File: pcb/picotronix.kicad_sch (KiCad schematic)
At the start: 27 parts, among them J1 Conn_02x04_Odd_Even, J2 Conn_02x04_Odd_Even, J3 DEBUG, J4 DB25_Male, U1 Pico, U2 LSF0204DPWR, U3 DAC7562SDGST, U4 ADA4891-3

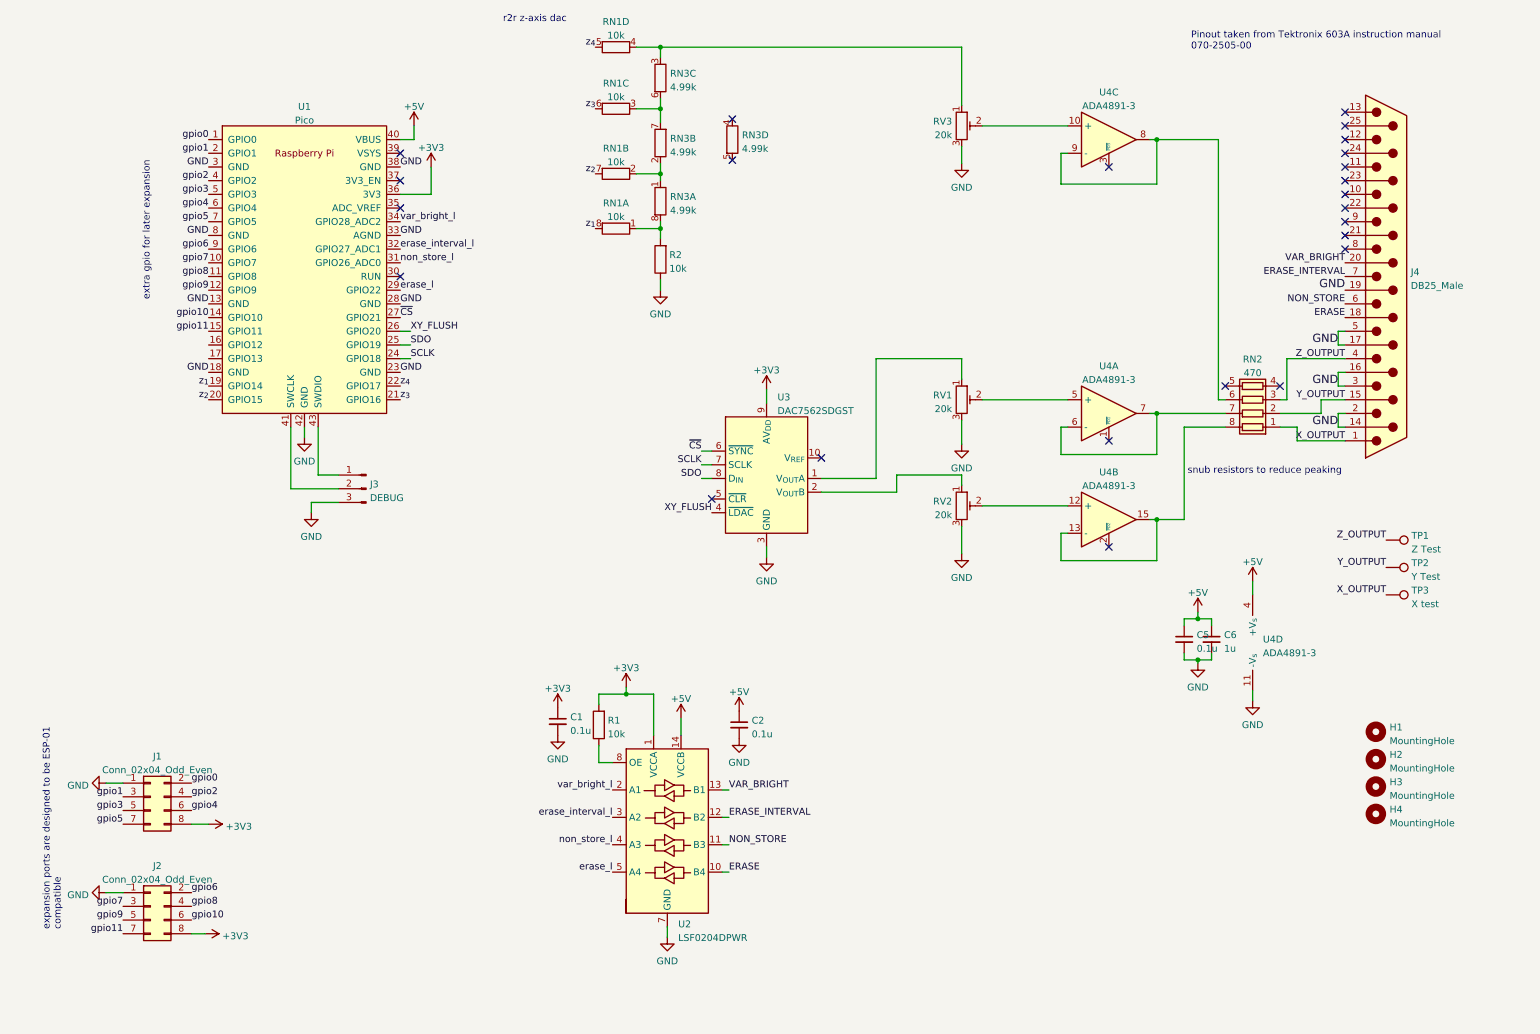
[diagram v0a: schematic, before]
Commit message: pcb rev2 routed
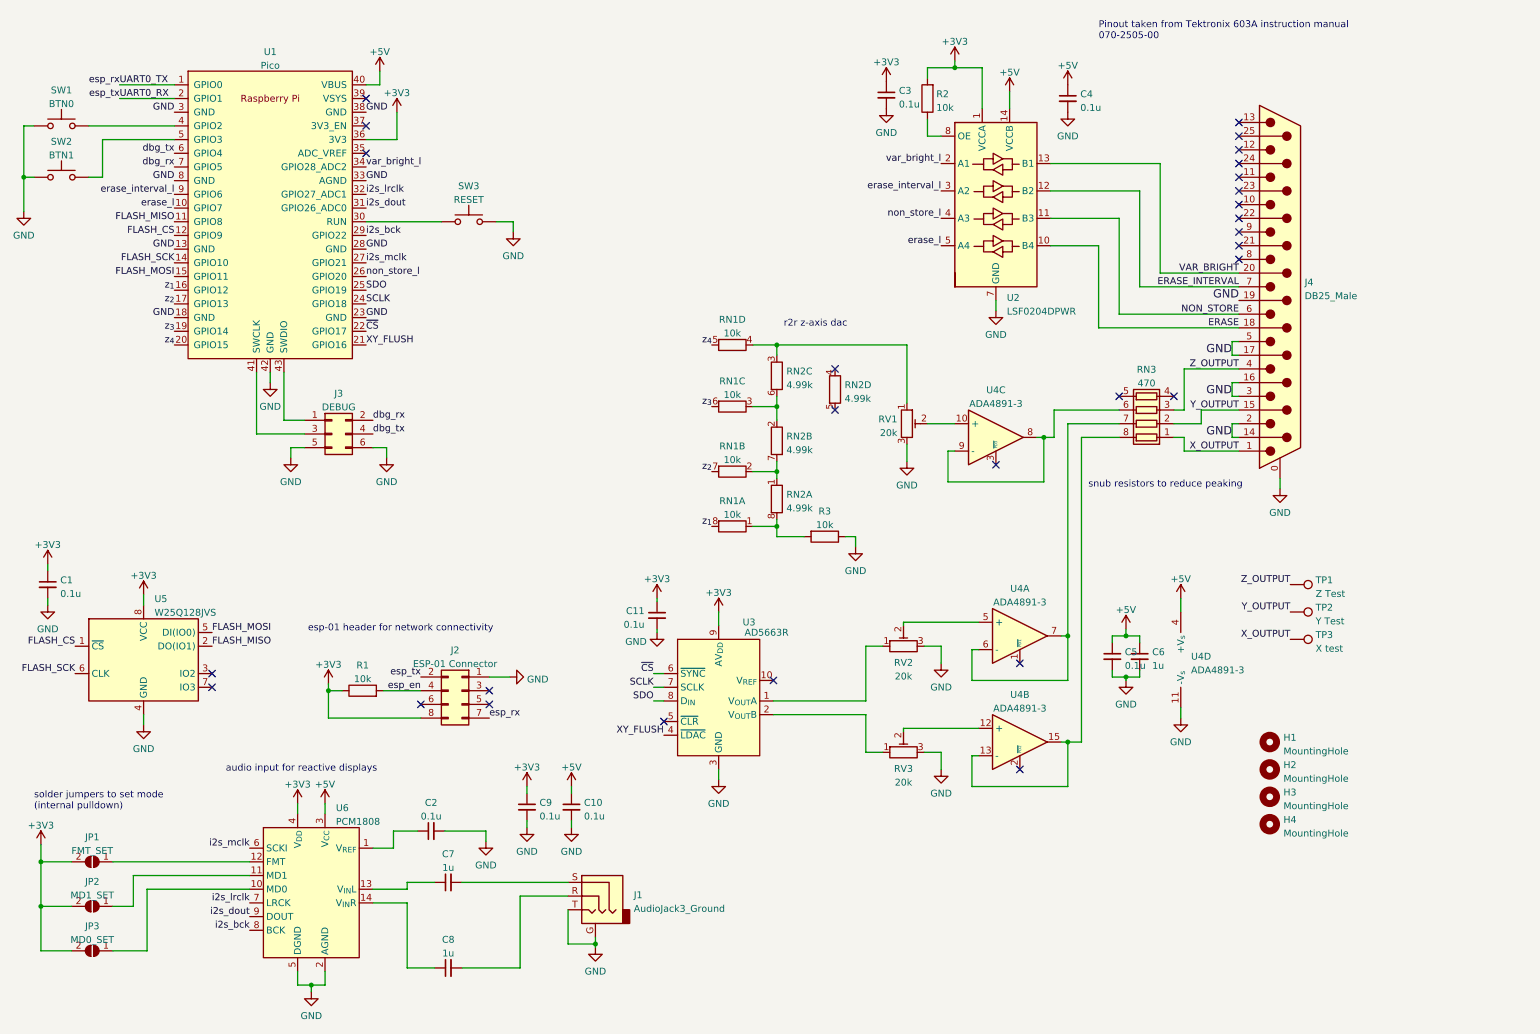
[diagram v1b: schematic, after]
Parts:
- removed J2: Conn_02x04_Odd_Even, Connector_PinSocket_2.54mm:PinSocket_2x04_P2.54mm_Vertical, symbol Connector_Generic:Conn_02x04_Odd_Even
- removed J3: DEBUG, Connector_PinHeader_2.54mm:PinHeader_1x03_P2.54mm_Vertical, symbol Connector:Conn_01x03_Male
- added C1, C10, C11, C2, C9: 0.1u, Capacitor_SMD:C_0603_1608Metric_Pad1.08x0.95mm_HandSolder, symbol Device:C_Small
- added C7, C8: 1u, Capacitor_SMD:C_0603_1608Metric_Pad1.08x0.95mm_HandSolder, symbol Device:C_Small
- added J1: AudioJack3_Ground, Connector_Audio:Jack_3.5mm_CUI_SJ-3524-SMT_Horizontal, symbol Connector:AudioJack3_Ground
- added J3: DEBUG, Connector_PinHeader_2.54mm:PinHeader_2x03_P2.54mm_Vertical, symbol Connector_Generic:Conn_02x03_Odd_Even
- added JP1: FMT_SET, Jumper:SolderJumper-2_P1.3mm_Open_TrianglePad1.0x1.5mm, symbol Jumper:SolderJumper_2_Open
- added JP2: MD1_SET, Jumper:SolderJumper-2_P1.3mm_Open_TrianglePad1.0x1.5mm, symbol Jumper:SolderJumper_2_Open
- added JP3: MD0_SET, Jumper:SolderJumper-2_P1.3mm_Open_TrianglePad1.0x1.5mm, symbol Jumper:SolderJumper_2_Open
- added R1: 10k, Resistor_SMD:R_0603_1608Metric_Pad0.98x0.95mm_HandSolder, symbol Device:R
- added SW1: BTN0, Button_Switch_SMD:SW_SPST_TL3305A, symbol Switch:SW_Push
- added SW2: BTN1, Button_Switch_SMD:SW_SPST_TL3305A, symbol Switch:SW_Push
- added SW3: RESET, Button_Switch_SMD:SW_SPST_TL3305A, symbol Switch:SW_Push
- added U5: W25Q128JVS, Package_SO:SOIC-8_5.23x5.23mm_P1.27mm, symbol Memory_Flash:W25Q128JVS
- added U6: PCM1808, Package_SO:TSSOP-14_4.4x5mm_P0.65mm, symbol picotronix:PCM1808
- J2: renamed from J1; value Conn_02x04_Odd_Even -> ESP-01 Connector
- J4: footprint Connector_Dsub:DSUB-25_Male_Horizontal_P2.77x2.54mm_EdgePinOffset9.40mm -> Connector_Dsub:DSUB-25_Male_Horizontal_P2.77x2.84mm_EdgePinOffset9.90mm_Housed_MountingHolesOffset11.32mm; symbol Connector:DB25_Male -> Connector:DB25_Male_MountingHoles
- TP1, TP2, TP3: footprint (none) -> TestPoint:TestPoint_Pad_2.0x2.0mm
- U3: value DAC7562SDGST -> AD5663R; footprint Package_SO:VSSOP-10_3x3mm_P0.5mm -> Package_SO:MSOP-10_3x3mm_P0.5mm; symbol picotronix:DAC7562SDGST -> picotronix:AD5663R; Digikey_PN 296-38921-1-ND -> AD5623RBRMZ-5REEL7CT-ND
- renumbered C1 to C3, C2 to C4, R1 to R2, R2 to R3, RN3 to RN2, RN2 to RN3, RV3 to RV1, RV1 to RV2, RV2 to RV3
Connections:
- net gpio6 is gone; now on net erase_interval_l: U1.9 (GPIO6)
- net gpio7 is gone; now on net erase_l: U1.10 (GPIO7)
- net +3V3: now also C1.1, C11.1, C9.1, JP1.2 (B), JP2.2 (B), JP3.2 (B), R1.1, U5.8 (VCC), U6.4 (V_{DD})
- net +5V: now also C10.1, U6.3 (V_{CC})
- net GND: now also J4.0 (PAD), C1.2, C10.2, C11.2, C2.2, C9.2, J1.G, J1.T, J3.5 (Pin_5), J3.6 (Pin_6), SW1.1, SW2.1, SW3.2, U5.4 (GND), U6.2 (AGND), U6.5 (DGND)
- net XY_FLUSH: now also U1.21 (GPIO16); no longer U1.26 (GPIO20)
- net erase_interval_l: no longer U1.32 (GPIO27_ADC1)
- net erase_l: no longer U1.29 (GPIO22)
- net non_store_l: now also U1.26 (GPIO20); no longer U1.31 (GPIO26_ADC0)
- net z_{1}: now also U1.16 (GPIO12); no longer U1.19 (GPIO14)
- net z_{2}: now also U1.17 (GPIO13); no longer U1.20 (GPIO15)
- net z_{3}: now also U1.19 (GPIO14); no longer U1.21 (GPIO16)
- net z_{4}: now also U1.20 (GPIO15); no longer U1.22 (GPIO17)
- net ~{CS}: now also U1.22 (GPIO17); no longer U1.27 (GPIO21)
- net at RN1.3 (R3.1), RN2.6 (R3.2): now also RN2.2 (R2.1); no longer RN2.7 (R2.2)
- net at RN1.2 (R2.1), RN2.1 (R1.1): now also RN2.7 (R2.2); no longer RN2.2 (R2.1)
- net at U1.30 (RUN): now also SW3.1
- net at U1.41 (SWCLK): now also J3.3 (Pin_3)
- net at U1.43 (SWDIO): now also J3.1 (Pin_1)
- net gpio0 renamed UART0_RX
- net UART0_RX: now also U1.2 (GPIO1); no longer U1.1 (GPIO0)
- net gpio1: no longer names the net of J2.3 (Pin_3)
- net gpio1: no longer U1.2 (GPIO1)
- net gpio10 renamed FLASH_SCK
- net FLASH_SCK: now also U5.6 (CLK)
- net gpio11 renamed FLASH_MOSI
- net FLASH_MOSI: now also U5.5 (DI(IO0))
- net gpio2: no longer names the net of U1.4 (GPIO2)
- net gpio2: now also SW1.2; no longer J2.4 (Pin_4)
- net gpio3: no longer names the net of J2.5 (Pin_5)
- net gpio3: no longer U1.5 (GPIO3)
- net gpio4: no longer names the net of J2.6 (Pin_6)
- net gpio4: no longer U1.6 (GPIO4)
- net gpio5 renamed UART0_TX
- net UART0_TX: now also U1.1 (GPIO0); no longer U1.7 (GPIO5)
- net gpio8 renamed FLASH_MISO
- net FLASH_MISO: now also U5.2 (DO(IO1))
- net gpio9 renamed FLASH_CS
- net FLASH_CS: now also U5.1 (~{CS})
- new net: JP2.1 (A), U6.11 (MD1)
- new net: JP3.1 (A), U6.10 (MD0)
- new net: SW2.2, U1.5 (GPIO3)
- new net: C2.1, U6.1 (V_{REF})
- new net: JP1.1 (A), U6.12 (FMT)
- new net: C7.1, U6.13 (V_{IN}L)
- new net: C8.1, U6.14 (V_{IN}R)
- new net: C7.2, J1.S
- new net: C8.2, J1.R
- new net dbg_rx: J3.2 (Pin_2), U1.7 (GPIO5)
- new net dbg_tx: J3.4 (Pin_4), U1.6 (GPIO4)
- new net esp_en: J2.4 (Pin_4), R1.2
- new net i2s_bck: U1.29 (GPIO22), U6.8 (BCK)
- new net i2s_dout: U1.31 (GPIO26_ADC0), U6.9 (DOUT)
- new net i2s_lrclk: U1.32 (GPIO27_ADC1), U6.7 (LRCK)
- new net i2s_mclk: U1.27 (GPIO21), U6.6 (SCKI)
- no-connect marks 24 -> 28
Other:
- note added: "audio input for reactive displays"
- note added: "esp-01 header for network connectivity"
- note added: "solder jumpers to set mode (internal pulldown)"
- note removed: "expansion ports are designed to be ESP-01 compatible"
- note removed: "extra gpio for later expansion"
- company: (none) -> Saji Champlin
- title: (none) -> Picotronix Main Board
- moved on the sheet: C3, C4, C5, C6, H1, H2, H3, H4, J2, R2, R3, RN1A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
